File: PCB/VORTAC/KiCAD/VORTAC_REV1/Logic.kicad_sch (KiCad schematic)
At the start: 26 parts, among them Q3 BSS138AKDW, U1 TLV73333PDBV, U3 EE-SX4320, U5 AS5047D, U6 AP63205WU, U7 EE-SX3350

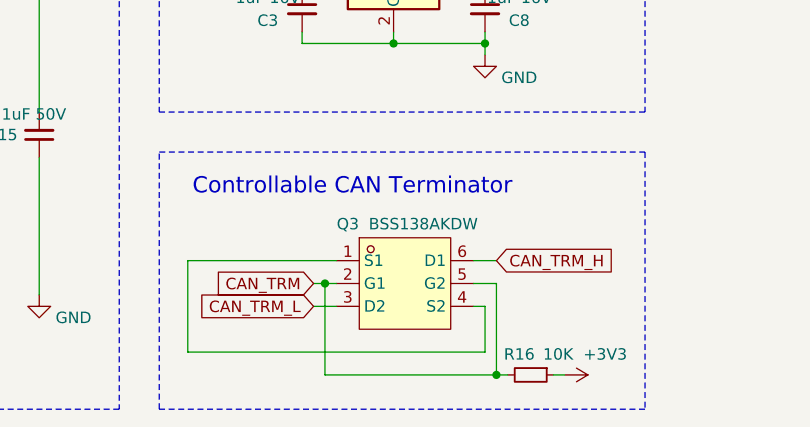
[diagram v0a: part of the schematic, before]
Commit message: Girl Math
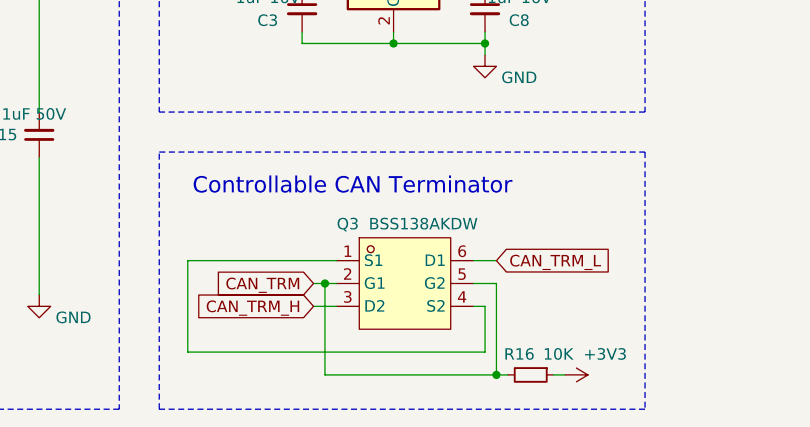
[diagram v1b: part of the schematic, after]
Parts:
- C30, C31: footprint Capacitor_SMD:C_0805_2012Metric -> Capacitor_SMD:C_0603_1608Metric
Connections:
- net CAN_TRM_H: now also Q3.3 (D2); no longer Q3.6 (D1)
- net CAN_TRM_L: now also Q3.6 (D1); no longer Q3.3 (D2)
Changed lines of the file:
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@@
 	(global_label "CAN_TRM_H"
 		(shape input)
-		(at 123.19 176.53 0)
+		(at 102.87 181.61 180)
 		(effects
 			(font
 				(size 1.27 1.27)
 			)
-			(justify left)
+			(justify right)
 		)
 		(property "Intersheetrefs" "${INTERSHEET_REFS}"
-			(at 123.19 176.53 0)
+			(at 102.87 181.61 0)
 			(effects
 				(font
@@
 	(global_label "CAN_TRM_L"
 		(shape input)
-		(at 102.87 181.61 180)
+		(at 123.19 176.53 0)
 		(effects
 			(font
 				(size 1.27 1.27)
 			)
-			(justify right)
+			(justify left)
 		)
 		(property "Intersheetrefs" "${INTERSHEET_REFS}"
-			(at 102.87 181.61 0)
+			(at 123.19 176.53 0)
 			(effects
 				(font
@@
 			)
 		)
-		(property "Footprint" "Capacitor_SMD:C_0805_2012Metric"
+		(property "Footprint" "Capacitor_SMD:C_0603_1608Metric"
 			(at 100.33 102.87 0)
 			(effects
@@
 			)
 		)
-		(property "Footprint" "Capacitor_SMD:C_0805_2012Metric"
+		(property "Footprint" "Capacitor_SMD:C_0603_1608Metric"
 			(at 114.3 102.87 0)
 			(effects

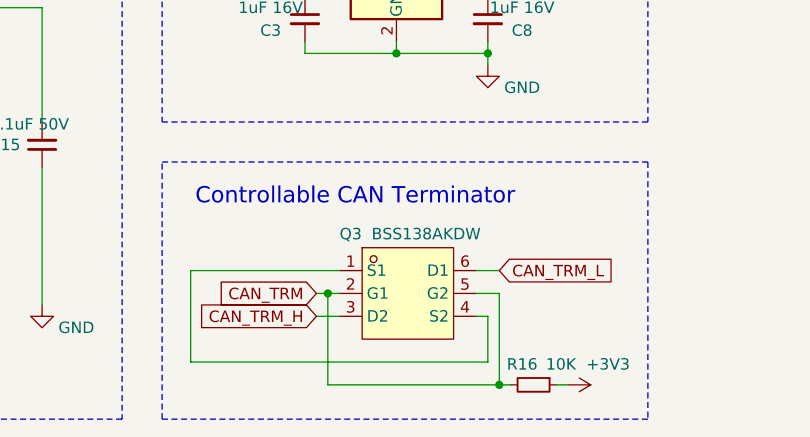
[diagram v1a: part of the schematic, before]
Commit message: Route me like one of you French girls
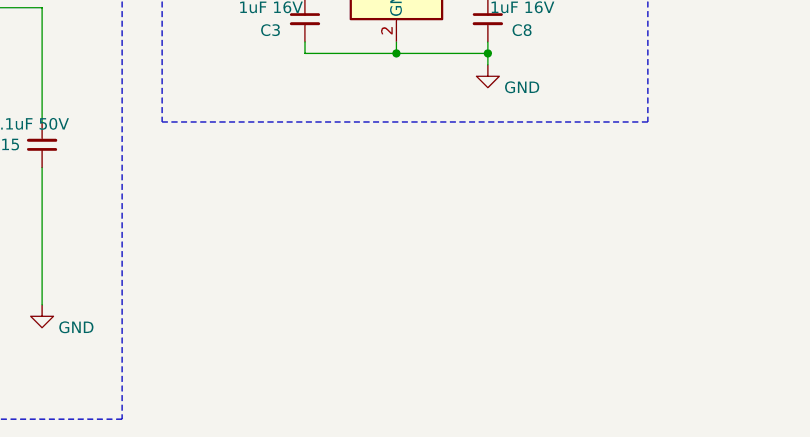
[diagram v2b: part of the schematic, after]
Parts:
- removed Q3: BSS138AKDW, Package_TO_SOT_SMD:SOT-363_SC-70-6, symbol Vortac:BSS138AKDW
- removed R16: 10K, Resistor_SMD:R_0402_1005Metric, symbol Device:R_Small
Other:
- note removed: "Controllable CAN Terminator"

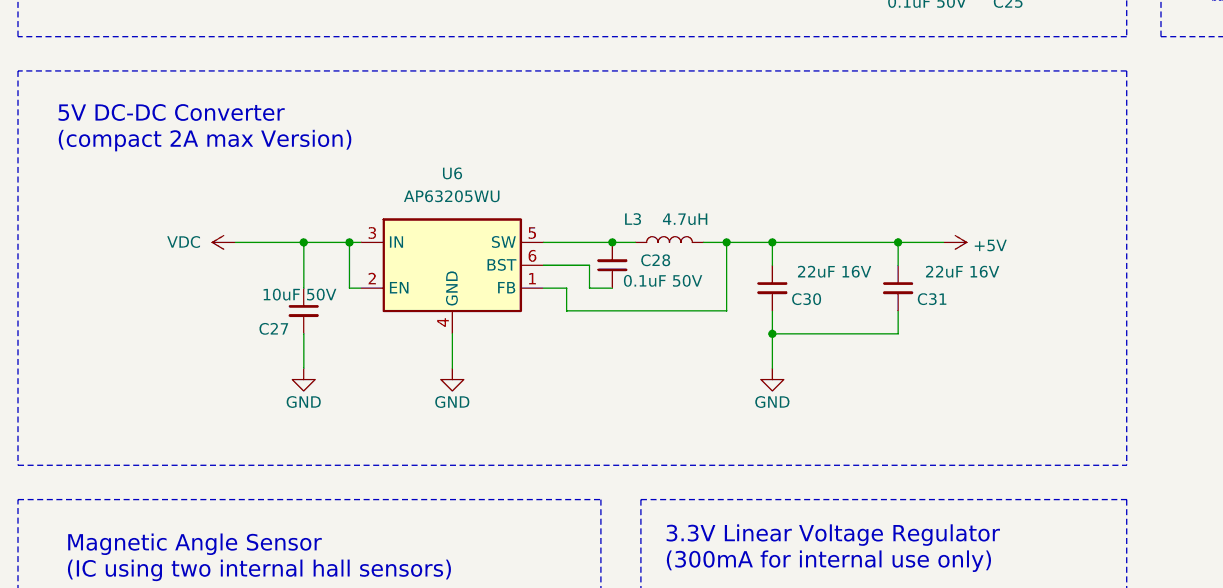
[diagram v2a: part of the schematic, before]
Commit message: I NEED A HEEEROOO
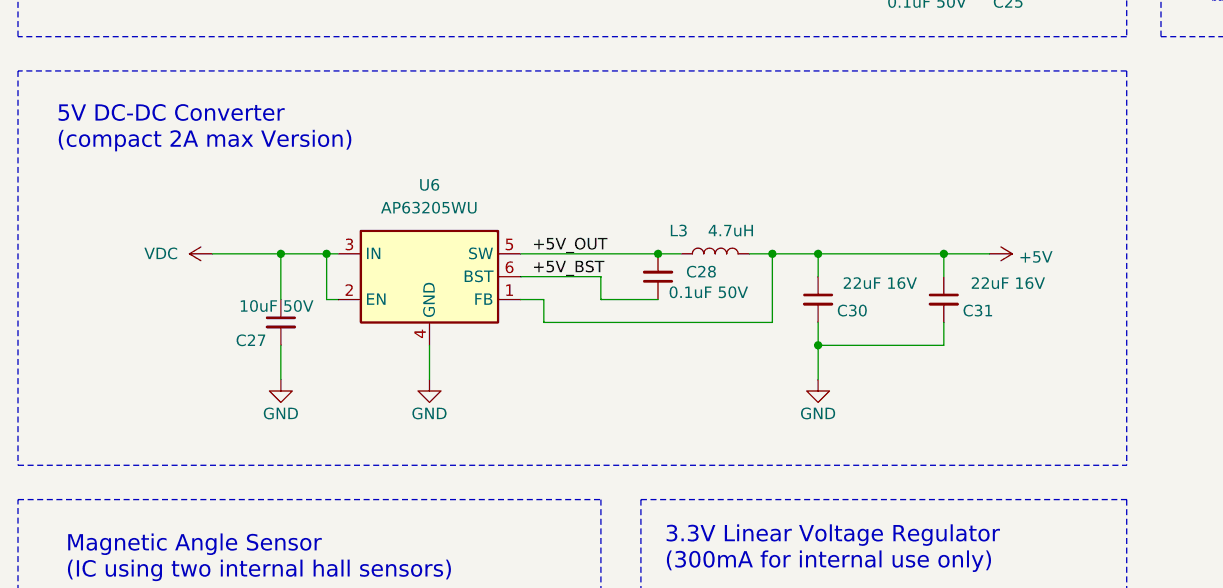
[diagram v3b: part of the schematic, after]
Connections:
- net +5V_OUT: now reaches C28.2, L3.1, U6.5 (SW)
- net +5V_BST: now reaches C28.1, U6.6 (BST)
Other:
- moved on the sheet: C27, C28, C30, C31, L3, U6

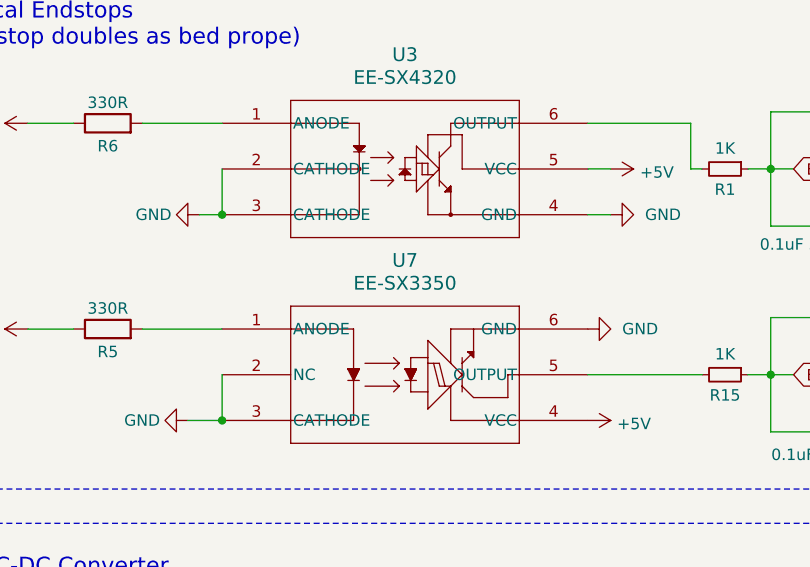
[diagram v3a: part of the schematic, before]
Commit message: KONGSTRONG
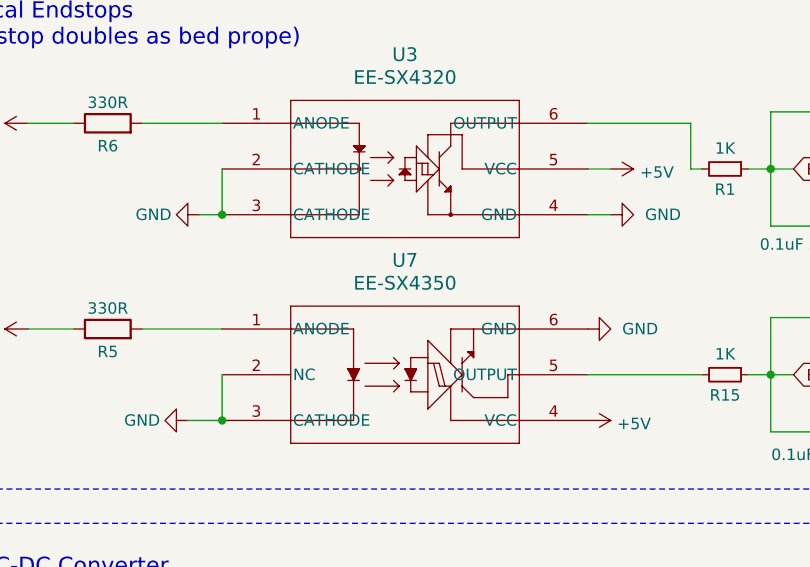
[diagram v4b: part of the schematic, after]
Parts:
- U7: value EE-SX3350 -> EE-SX4350; LCSC C7470740 -> C17524058
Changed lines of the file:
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@@
 			)
 		)
-		(property "Value" "EE-SX3350"
+		(property "Value" "EE-SX4350"
 			(at 72.39 52.07 0)
 			(effects
@@
 			)
 		)
-		(property "LCSC" "C7470740"
+		(property "LCSC" "C17524058"
 			(at 52.07 57.15 0)
 			(effects
